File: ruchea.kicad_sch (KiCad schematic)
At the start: 22 parts, among them J11 Conn_01x04, J12 Conn_01x04, J17 Conn_01x04, J18 Conn_01x04, J4 Conn_01x02, J5 Conn_01x04, J8 Conn_01x02, Q6 PMBT2222A,215, U4 TCA9548APWR, U7 1043

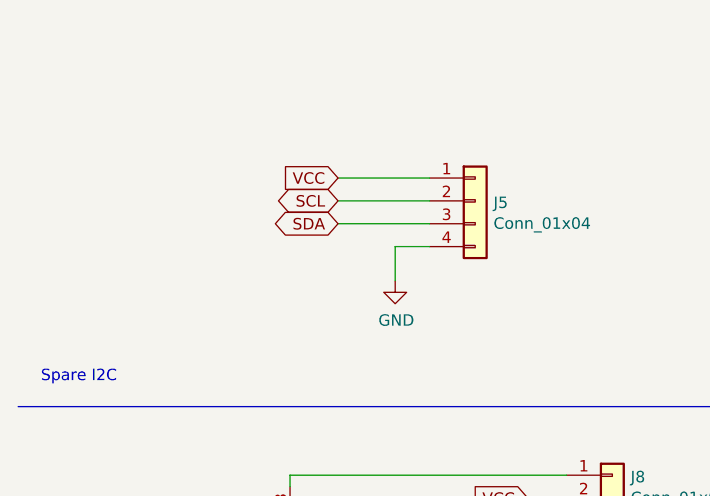
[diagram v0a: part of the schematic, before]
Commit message: Update
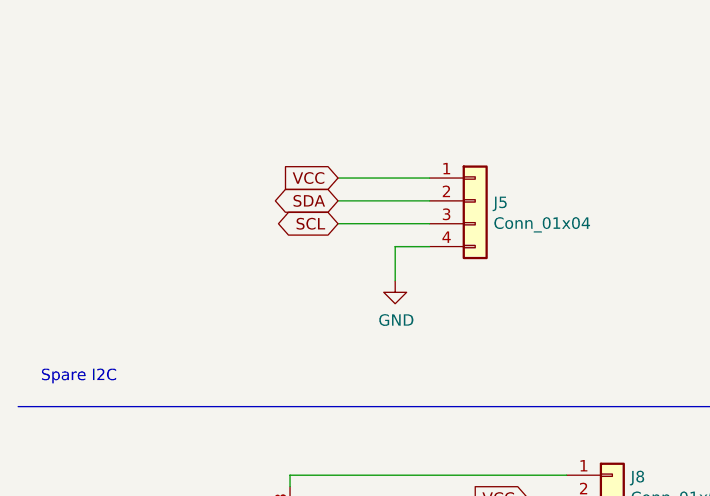
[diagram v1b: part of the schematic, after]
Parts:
- J11, J12, J17, J18: footprint Connector_JST:JST_PH_B4B-PH-K_1x04_P2.00mm_Vertical -> Empreintes:1725672
- J5: footprint Empreintes:1989764 -> Empreintes:1725672
- J8: footprint Empreintes:1989748 -> Empreintes:1725656
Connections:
- net SCL: now also J5.3 (Pin_3); no longer J5.2 (Pin_2)
- net SDA: now also J5.2 (Pin_2); no longer J5.3 (Pin_3)
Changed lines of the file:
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@@
 	(global_label "SCL"
 		(shape bidirectional)
-		(at 48.26 33.02 180)
+		(at 48.26 35.56 180)
 		(fields_autoplaced yes)
 		(effects
@@
 		)
 		(property "Intersheetrefs" "${INTERSHEET_REFS}"
-			(at -199.39 -67.31 0)
+			(at -199.39 -64.77 0)
 			(effects
 				(font
@@
 	(global_label "SDA"
 		(shape bidirectional)
-		(at 48.26 35.56 180)
+		(at 48.26 33.02 180)
 		(fields_autoplaced yes)
 		(effects
@@
 		)
 		(property "Intersheetrefs" "${INTERSHEET_REFS}"
-			(at -199.39 -67.31 0)
+			(at -199.39 -69.85 0)
 			(effects
 				(font
@@
 			)
 		)
-		(property "Footprint" "Connector_JST:JST_PH_B4B-PH-K_1x04_P2.00mm_Vertical"
+		(property "Footprint" "Empreintes:1725672"
 			(at 143.51 176.53 0)
 			(effects
@@
 			)
 		)
-		(property "Footprint" "Connector_JST:JST_PH_B4B-PH-K_1x04_P2.00mm_Vertical"
+		(property "Footprint" "Empreintes:1725672"
 			(at 265.43 142.24 0)
 			(effects
@@
 			)
 		)
-		(property "Footprint" "Empreintes:1989748"
+		(property "Footprint" "Empreintes:1725656"
 			(at 78.74 63.5 0)
 			(effects
@@
 			)
 		)
-		(property "Footprint" "Connector_JST:JST_PH_B4B-PH-K_1x04_P2.00mm_Vertical"
+		(property "Footprint" "Empreintes:1725672"
 			(at 143.51 139.7 0)
 			(effects
@@
 			)
 		)
-		(property "Footprint" "Connector_JST:JST_PH_B4B-PH-K_1x04_P2.00mm_Vertical"
+		(property "Footprint" "Empreintes:1725672"
 			(at 211.582 141.732 0)
 			(effects
@@
 			)
 		)
-		(property "Footprint" "Empreintes:1989764"
+		(property "Footprint" "Empreintes:1725672"
 			(at 63.5 33.02 0)
 			(effects

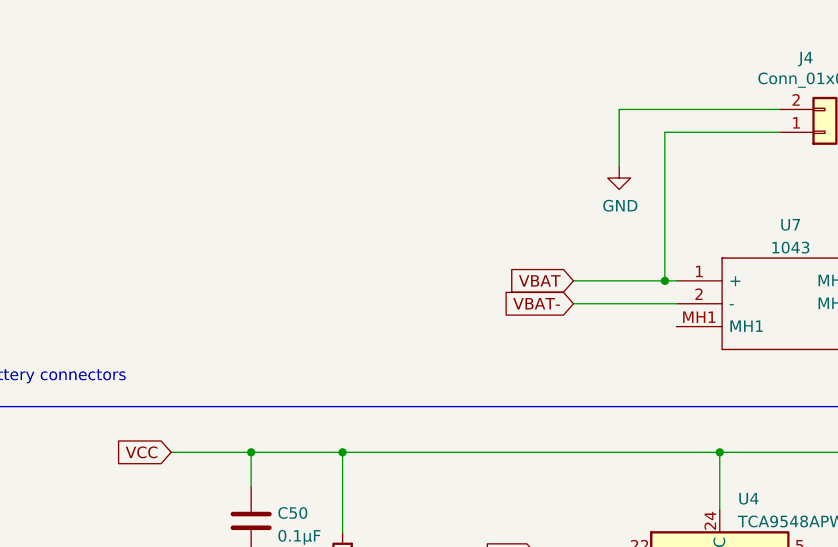
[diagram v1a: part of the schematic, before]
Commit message: update
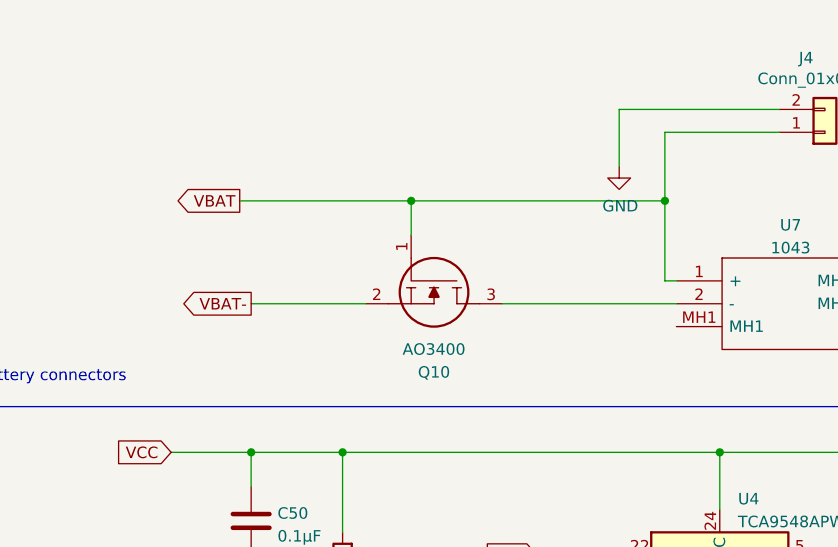
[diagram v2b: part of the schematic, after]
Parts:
- added Q10: AO3400, Package_TO_SOT_SMD:SOT-23, symbol AO3400:AO3400
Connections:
- net VBAT: now also Q10.1
- net VBAT-: now also Q10.2; no longer U7.2 (-)
- new net: Q10.3, U7.2 (-)
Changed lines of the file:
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@@
+	)
+	(junction
+		(at 149.86 33.02)
+		(diameter 0)
+		(color 0 0 0 0)
 	)
 	(junction
@@
 	)
 	(junction
-		(at 178.054 41.91)
-		(diameter 0)
-		(color 0 0 0 0)
-	)
-	(junction
 		(at 264.16 60.96)
 		(diameter 0)
@@
 	)
 	(junction
+		(at 178.054 33.02)
+		(diameter 0)
+		(color 0 0 0 0)
+	)
+	(junction
 		(at 264.16 92.71)
 		(diameter 0)
@@
 	(wire
 		(pts
-			(xy 178.054 41.91) (xy 178.054 25.4)
-		)
-		(stroke
-			(width 0)
-			(type default)
-		)
-	)
-	(wire
-		(pts
 			(xy 69.342 66.04) (xy 73.66 66.04)
 		)
@@
 	(wire
 		(pts
-			(xy 167.894 44.45) (xy 179.324 44.45)
+			(xy 132.08 44.45) (xy 144.78 44.45)
 		)
 		(stroke
@@
 	(wire
 		(pts
-			(xy 167.894 41.91) (xy 178.054 41.91)
+			(xy 130.81 33.02) (xy 149.86 33.02)
+		)
+		(stroke
+			(width 0)
+			(type default)
+		)
+	)
+	(wire
+		(pts
+			(xy 160.02 44.45) (xy 179.324 44.45)
 		)
 		(stroke
@@
 	(wire
 		(pts
+			(xy 178.054 33.02) (xy 178.054 41.91)
+		)
+		(stroke
+			(width 0)
+			(type default)
+		)
+	)
+	(wire
+		(pts
 			(xy 217.17 77.47) (xy 276.86 77.47)
 		)
@@
 		)
 	)
+	(wire
+		(pts
+			(xy 149.86 33.02) (xy 178.054 33.02)
+		)
+		(stroke
+			(width 0)
+			(type default)
+		)
+	)
 	(polyline
 		(pts
@@
 	(wire
 		(pts
+			(xy 178.054 33.02) (xy 178.054 25.4)
+		)
+		(stroke
+			(width 0)
+			(type default)
+		)
+	)
+	(wire
+		(pts
 			(xy 217.17 69.85) (xy 217.17 77.47)
 		)
@@
 		(pts
 			(xy 167.64 102.87) (xy 173.99 102.87)
+		)
+		(stroke
+			(width 0)
+			(type default)
+		)
+	)
+	(wire
+		(pts
+			(xy 149.86 33.02) (xy 149.86 36.83)
 		)
 		(stroke
@@
 	)
 	(global_label "VBAT-"
-		(shape input)
-		(at 167.894 44.45 180)
+		(shape output)
+		(at 132.08 44.45 180)
 		(fields_autoplaced yes)
 		(effects
@@
 		)
 		(property "Intersheetrefs" "${INTERSHEET_REFS}"
-			(at 159.5827 44.3706 0)
+			(at 123.7618 44.45 0)
 			(effects
 				(font
@@
 	)
 	(global_label "VBAT"
-		(shape input)
-		(at 167.894 41.91 180)
-		(fields_autoplaced yes)
+		(shape output)
+		(at 130.81 33.02 180)
 		(effects
 			(font
@@
 		)
 		(property "Intersheetrefs" "${INTERSHEET_REFS}"
-			(at 161.155 41.8306 0)
+			(at 108.831 20.2406 0)
 			(effects
 				(font
@@
 					(unit 1)
 				)
+			)
+		)
+	)
+	(symbol
+		(lib_id "AO3400:AO3400")
+		(at 149.86 36.83 270)
+		(unit 1)
+		(exclude_from_sim no)
+		(in_bom yes)
+		(on_board yes)
+		(dnp no)
+		(property "Reference" "Q10"
+			(at 152.4 52.07 90)
+			(effects
+				(font
+					(size 1.27 1.27)
+				)
+			)
+		)
+		(property "Value" "AO3400"
+			(at 152.4 49.53 90)
+			(effects
+				(font
+					(size 1.27 1.27)
+				)
+			)
+		)
+		(property "Footprint" "Package_TO_SOT_SMD:SOT-23"
+			(at 148.59 48.26 0)
+			(effects
+				(font
+					(size 1.27 1.27)
+				)
+				(justify left)
+				(hide yes)
+			)
+		)
+		(property "Datasheet" "http://aosmd.com/res/data_sheets/AO3400.pdf"
+			(at 146.05 48.26 0)
+			(effects
+				(font
+					(size 1.27 1.27)
+				)
+				(justify left)
+				(hide yes)
+			)
+		)
+		(property "Description" ""
+			(at 149.86 36.83 0)
+			(effects
+				(font
+					(size 1.27 1.27)
+				)
+				(hide yes)
+			)
+		)
+		(property "Description_1" "30V N-Channel MOSFET"
+			(at 143.51 48.26 0)
+			(effects
+				(font
+					(size 1.27 1.27)
+				)
+				(justify left)
+				(hide yes)
+			)
+		)
+		(property "Height" "1.25"
+			(at 140.97 48.26 0)
+			(effects
+				(font
+					(size 1.27 1.27)
+				)
+				(justify left)
+				(hide yes)
+			)
+		)
+		(property "Manufacturer_Name" "Alpha & Omega Semiconductors"
+			(at 138.43 48.26 0)
+			(effects
+				(font
+					(size 1.27 1.27)
+				)
+				(justify left)
+				(hide yes)
+			)
+		)
+		(property "Manufacturer_Part_Number" "AO3400"
+			(at 135.89 48.26 0)
+			(effects
+				(font
+					(size 1.27 1.27)
+				)
+				(justify left)
+				(hide yes)
+			)
+		)
+		(property "Mouser Part Number" ""
+			(at 133.35 48.26 0)
+			(effects
+				(font
+					(size 1.27 1.27)
+				)
+				(justify left)
+				(hide yes)
+			)
+		)
+		(property "Mouser Price/Stock" ""
+			(at 130.81 48.26 0)
+			(effects
+				(font
+					(size 1.27 1.27)
+				)
+				(justify left)
+				(hide yes)
+			)
+		)
+		(property "Arrow Part Number" "AO3400"
+			(at 128.27 48.26 0)
+			(effects
+				(font
+					(size 1.27 1.27)
+				)
+				(justify left)
+				(hide yes)
+			)
+		)
+		(property "Arrow Price/Stock" "https://www.arrow.com/en/products/ao3400/alpha-and-omega-semiconductor"
+			(at 125.73 48.26 0)
+			(effects
+				(font
+					(size 1.27 1.27)
+				)
+				(justify left)
+				(hide yes)
+			)
+		)
+		(pin "2"
+		)
+		(pin "3"
+		)
+		(pin "1"
+		)
+		(instances
+			(project ""
+				(path "/a4bf92fd-0992-4ef9-a190-19a629782be3/00000000-0000-0000-0000-00006011445d"
+					(reference "Q10")
+					(unit 1)
+				)
